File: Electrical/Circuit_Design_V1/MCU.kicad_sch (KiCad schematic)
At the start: 10 parts, among them U1 STM32G474RETx

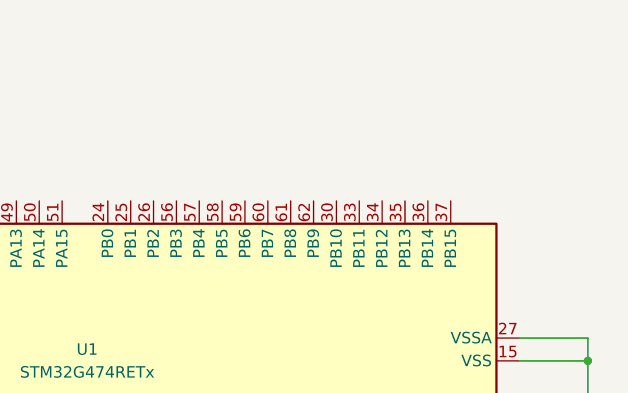
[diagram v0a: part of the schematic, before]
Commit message: #3 Finishing some circuitry.
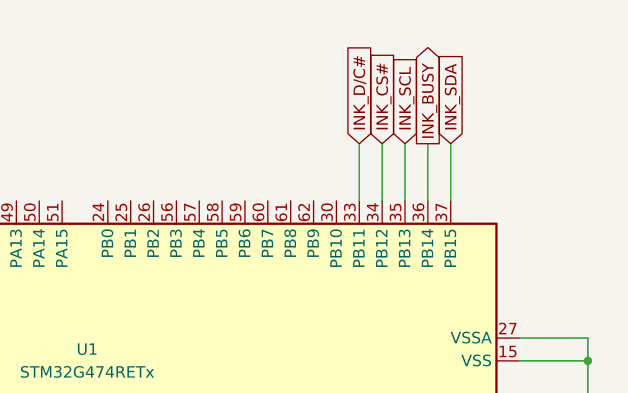
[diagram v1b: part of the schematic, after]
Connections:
- net INK_D/C#: now reaches U1.33 (PB11)
- net INK_CS#: now reaches U1.34 (PB12)
- net INK_SCL: now reaches U1.35 (PB13)
- net INK_BUSY: now reaches U1.36 (PB14)
- net INK_SDA: now reaches U1.37 (PB15)
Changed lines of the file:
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@@
+	(wire
+		(pts
+			(xy 180.34 55.88) (xy 180.34 62.23)
+		)
+		(stroke
+			(width 0)
+			(type default)
+		)
+	)
 	(wire
 		(pts
@@
 	(wire
 		(pts
+			(xy 182.88 55.88) (xy 182.88 62.23)
+		)
+		(stroke
+			(width 0)
+			(type default)
+		)
+	)
+	(wire
+		(pts
 			(xy 49.53 161.29) (xy 49.53 156.21)
 		)
@@
 	(wire
 		(pts
+			(xy 187.96 55.88) (xy 187.96 62.23)
+		)
+		(stroke
+			(width 0)
+			(type default)
+		)
+	)
+	(wire
+		(pts
 			(xy 92.71 77.47) (xy 101.6 77.47)
 		)
@@
 	(wire
 		(pts
+			(xy 185.42 55.88) (xy 185.42 62.23)
+		)
+		(stroke
+			(width 0)
+			(type default)
+		)
+	)
+	(wire
+		(pts
 			(xy 74.93 62.23) (xy 69.85 62.23)
 		)
@@
 		(pts
 			(xy 144.78 97.79) (xy 144.78 101.6)
+		)
+		(stroke
+			(width 0)
+			(type default)
+		)
+	)
+	(wire
+		(pts
+			(xy 190.5 55.88) (xy 190.5 62.23)
 		)
 		(stroke
@@
 		)
 	)
+	(global_label "INK_SCL"
+		(shape input)
+		(at 185.42 55.88 90)
+		(fields_autoplaced yes)
+		(effects
+			(font
+				(size 1.27 1.27)
+			)
+			(justify left)
+		)
+		(property "Intersheetrefs" "${INTERSHEET_REFS}"
+			(at 185.42 45.2143 90)
+			(effects
+				(font
+					(size 1.27 1.27)
+				)
+				(justify left)
+				(hide yes)
+			)
+		)
+	)
 	(global_label "ADX_SCLK"
 		(shape input)
@@
 		)
 	)
+	(global_label "INK_SDA"
+		(shape input)
+		(at 190.5 55.88 90)
+		(fields_autoplaced yes)
+		(effects
+			(font
+				(size 1.27 1.27)
+			)
+			(justify left)
+		)
+		(property "Intersheetrefs" "${INTERSHEET_REFS}"
+			(at 190.5 45.1538 90)
+			(effects
+				(font
+					(size 1.27 1.27)
+				)
+				(justify left)
+				(hide yes)
+			)
+		)
+	)
+	(global_label "INK_D{slash}C#"
+		(shape input)
+		(at 180.34 55.88 90)
+		(fields_autoplaced yes)
+		(effects
+			(font
+				(size 1.27 1.27)
+			)
+			(justify left)
+		)
+		(property "Intersheetrefs" "${INTERSHEET_REFS}"
+			(at 180.34 43.5814 90)
+			(effects
+				(font
+					(size 1.27 1.27)
+				)
+				(justify left)
+				(hide yes)
+			)
+		)
+	)
 	(global_label "ADX_INT1"
 		(shape output)
@@
 		)
 	)
+	(global_label "INK_CS#"
+		(shape input)
+		(at 182.88 55.88 90)
+		(fields_autoplaced yes)
+		(effects
+			(font
+				(size 1.27 1.27)
+			)
+			(justify left)
+		)
+		(property "Intersheetrefs" "${INTERSHEET_REFS}"
+			(at 182.88 44.9724 90)
+			(effects
+				(font
+					(size 1.27 1.27)
+				)
+				(justify left)
+				(hide yes)
+			)
+		)
+	)
 	(global_label "ADX_SDI"
 		(shape input)
@@
 			(effects
 				(font
+					(size 1.27 1.27)
+				)
+				(justify left)
+				(hide yes)
+			)
+		)
+	)
+	(global_label "INK_BUSY"
+		(shape output)
+		(at 187.96 55.88 90)
+		(fields_autoplaced yes)
+		(effects
+			(font
+				(size 1.27 1.27)
+			)
+			(justify left)
+		)
+		(property "Intersheetrefs" "${INTERSHEET_REFS}"
+			(at 187.96 43.8233 90)
+			(effects
+				(font
